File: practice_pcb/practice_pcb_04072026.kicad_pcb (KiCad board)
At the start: 4 copper layers, 61.5 x 44 mm, 19 parts, among them J1 VEE connector, J2 From_MCU, J3 MOSFET_out, J4 Conn_01x03, Q4 IRF3710, U5 NSi6651A

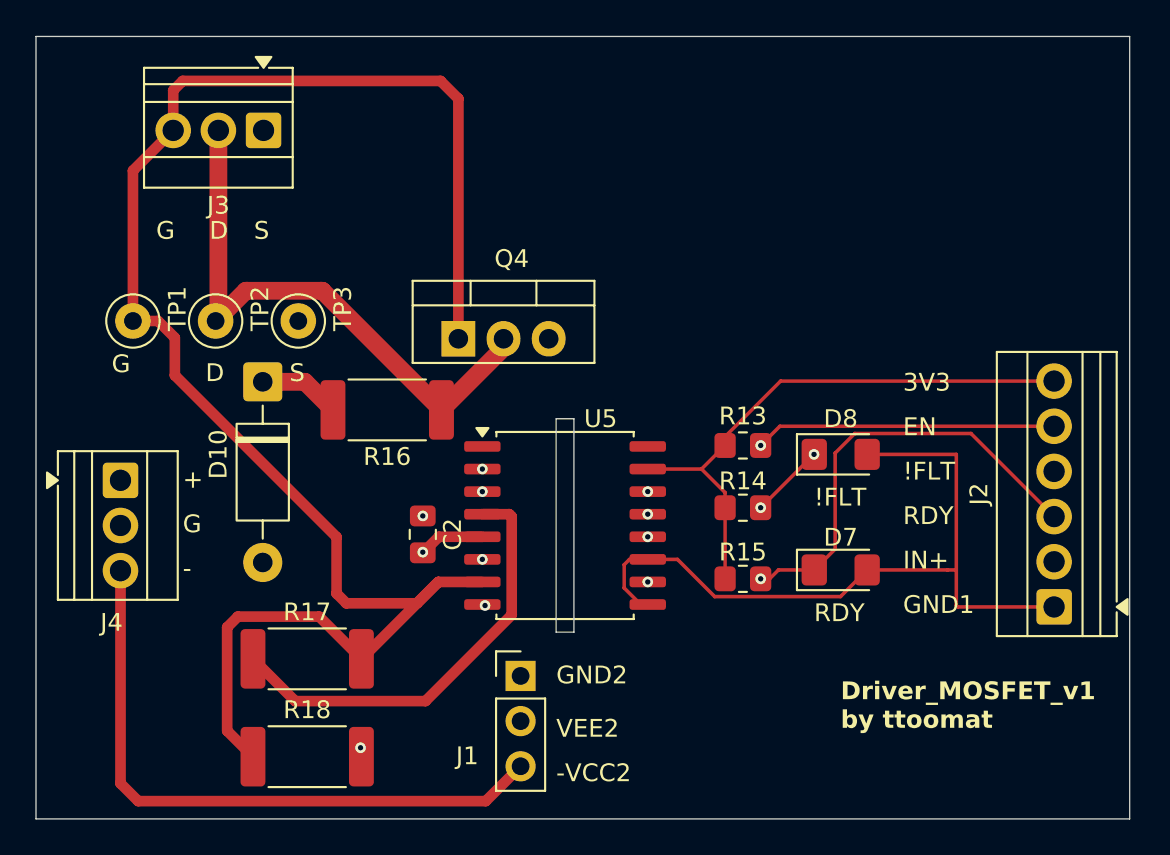
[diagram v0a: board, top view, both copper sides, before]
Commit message: Drive PCB remake.
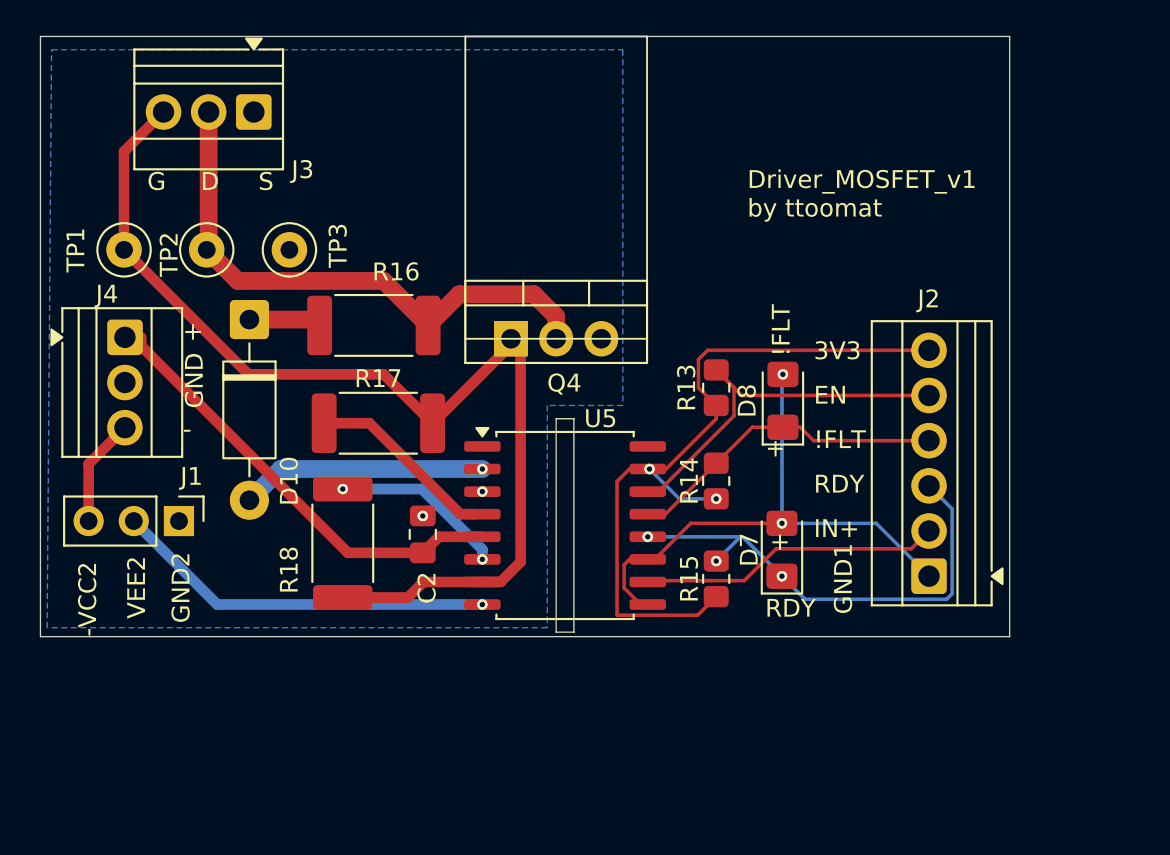
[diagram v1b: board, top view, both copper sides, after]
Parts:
- moved J1 21.1 mm to (91.8, 79.8), turned to -90 degrees
- moved R17 13.8 mm to (103.0, 74.2)
- moved R18 12.2 mm to (101.0, 81.0), turned to 90 degrees
- moved J4 8.04 mm to (88.8, 69.4)
- moved J2 7.24 mm to (134.0, 82.8)
- moved R16 4.81 mm to (102.8, 68.8)
- moved D8 4.43 mm to (125.8, 73.0), turned to 90 degrees
- moved TP1 4.03 mm to (88.7, 64.5)
- moved TP2 4.03 mm to (93.3, 64.5)
- moved TP3 4.03 mm to (98.0, 64.5)
- moved D10 3.58 mm to (95.8, 68.4)
- moved R13 3.58 mm to (122.0, 72.2), turned to 90 degrees
- moved D7 3.49 mm to (125.7, 81.4), turned to 90 degrees
- moved Q4 2.96 mm to (110.5, 69.5)
- moved R14 2.12 mm to (122.0, 77.5), turned to 90 degrees
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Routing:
- net Net-(J3-Pin_3): track 96.7 -> 61.5 mm
- net -15_DRV2: track 35.7 -> 6.09 mm
- net Net-(J1-Pin_2): track 7.33 -> 21.5 mm
- net Net-(U5-OUTH): track 24.8 -> 11.0 mm
- net GND_DRV1: track 42.4 -> 30.8 mm, vias 0 -> 2
- net +3V3_DRV1: track 31.9 -> 42.8 mm, vias 0 -> 2
- net Net-(J2-Pin_2): track 25.2 -> 17.0 mm, vias 1 -> 0
- net Net-(D8-K): track 24.7 -> 18.2 mm, vias 3 -> 0
- net Net-(D7-K): track 32.3 -> 27.4 mm, vias 2 -> 3
- net Net-(U5-OUTL): track 13.4 -> 9.81 mm
- net Net-(J2-Pin_5): track 24.4 -> 22.2 mm, vias 2 -> 0
- net +15_DRV2: track 24.5 -> 25.8 mm, vias 1 -> 0
- net /SINE (from OpAmp): track 32.6 -> 31.7 mm
- net Net-(D10-A): track 14.6 -> 13.8 mm
- net Net-(D10-K): track 4.60 -> 4.09 mm
- added copper zone on B.Cu, net GND_DRV2
- removed copper zone on In2.Cu, net GND_DRV2
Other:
- board size 61.5 x 44 mm -> 54.5 x 33.8 mm
- copper layers 4 -> 2
- board text added: "GND"
